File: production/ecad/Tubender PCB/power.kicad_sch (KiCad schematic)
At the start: 53 parts, among them Q1 CSD19502Q5B, Q2 CSD19534Q5A, U1 LMR36520FADDAR, U11 LM5146RGYR, U13 LM5017SDX/NOPB, U3 MCP23017-E_SO

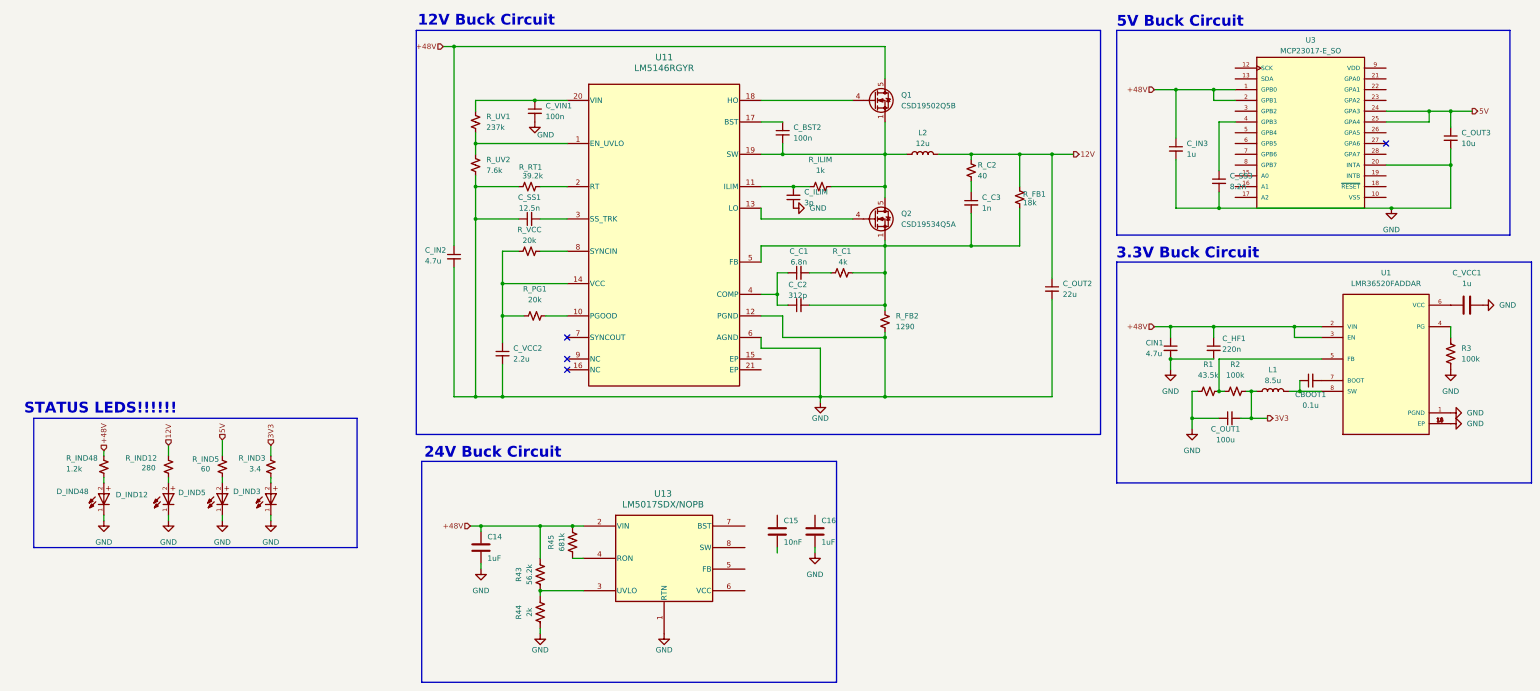
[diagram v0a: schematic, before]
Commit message: adjustments
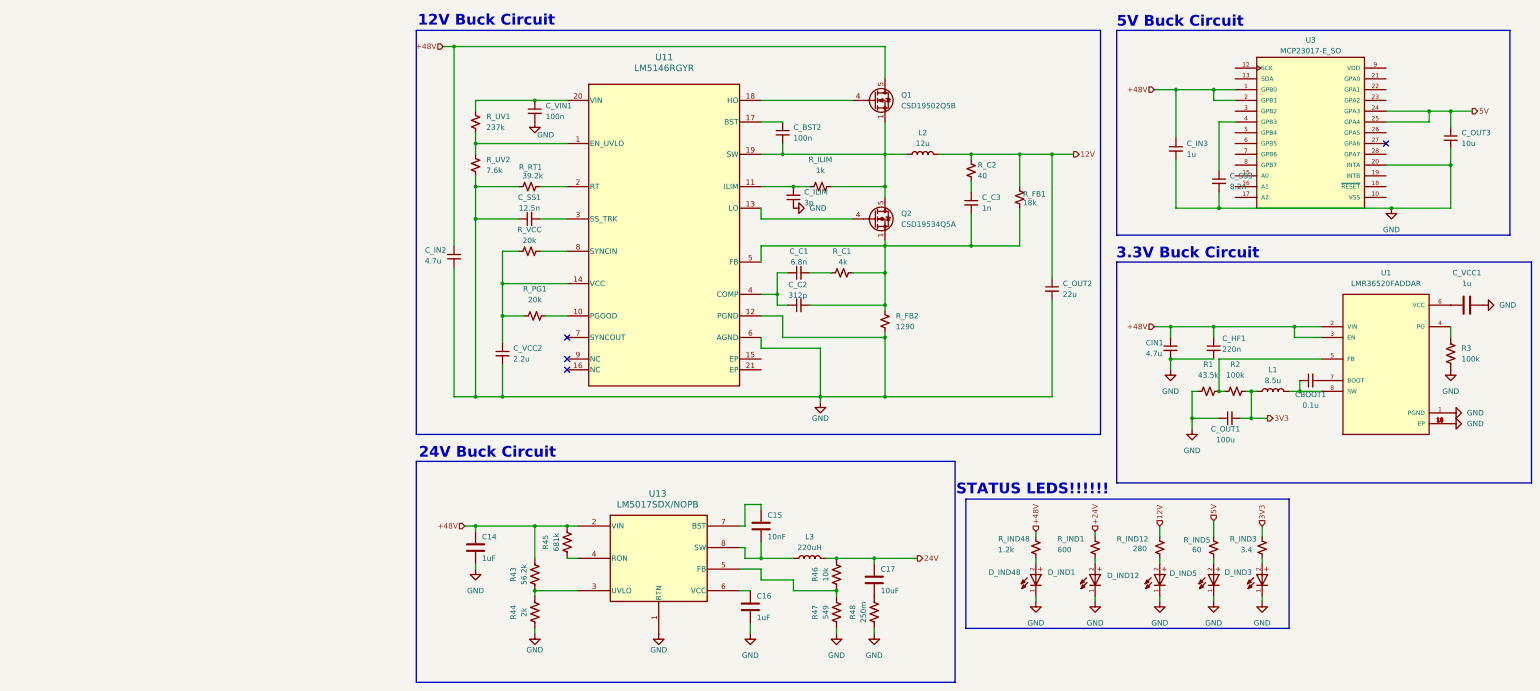
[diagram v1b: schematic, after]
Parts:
- added C17: 10uF, symbol Device:C
- added D_IND1: WL-SMCW_0603, WL-SMCW_0603:WL-SMCW_0603, symbol WL-SMCW_0603:WL-SMCW_0603
- added L3: 220uH, symbol Device:L
- added R46: 10k, symbol Device:R_US
- added R47: 549, symbol Device:R_US
- added R48: 250m, symbol Device:R_US
- added R_IND1: 600, symbol Device:R_Small_US
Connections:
- net GND: now also D_IND1.1, R47.1, R48.1
- net at C16.1: now also U13.6 (VCC)
- net at U13.5 (FB): now also R46.1, R47.2
- net at U13.7 (BST): now also C15.1
- net at U13.8 (SW): now also C15.2, L3.1
- new net: C17.2, R48.2
- new net: D_IND1.2, R_IND1.2
- new net +24V: R_IND1.1
- new net 24V: C17.1, L3.2, R46.2
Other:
- moved on the sheet: C14, C15, C16, D_IND12, D_IND3, D_IND48, D_IND5, R43, R44, R45, R_IND12, R_IND3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
